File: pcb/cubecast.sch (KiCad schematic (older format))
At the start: 17 parts, among them P1 TP, U1 bq24040, U2 tps62200, U3 ESP-07v2

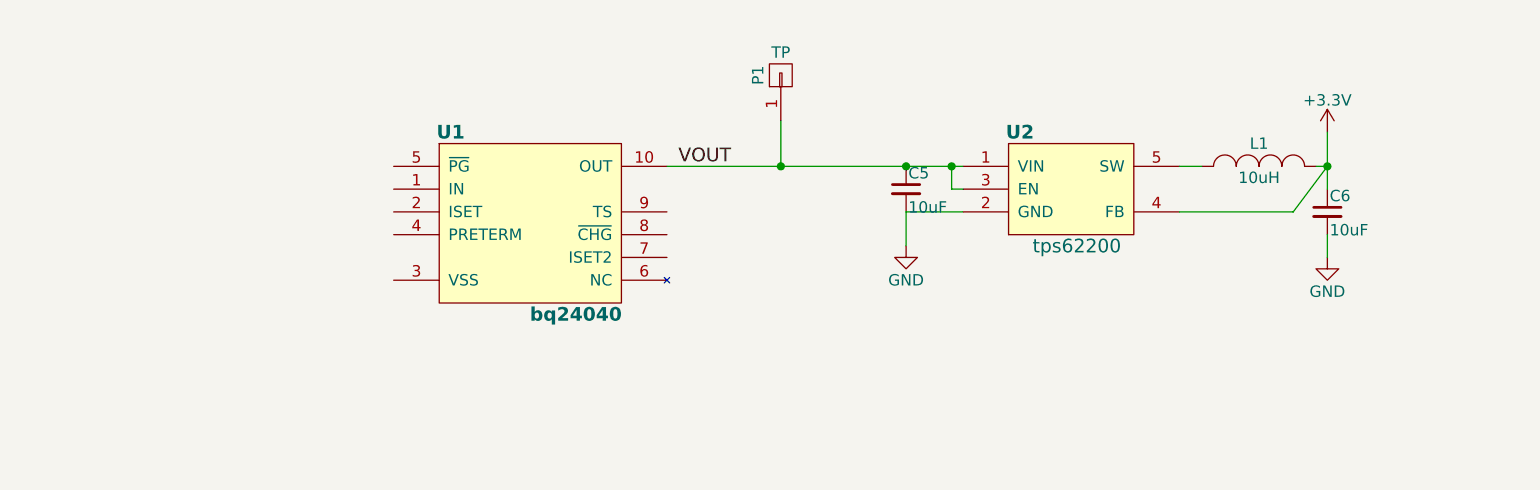
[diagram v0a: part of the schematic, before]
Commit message: footprint for charger
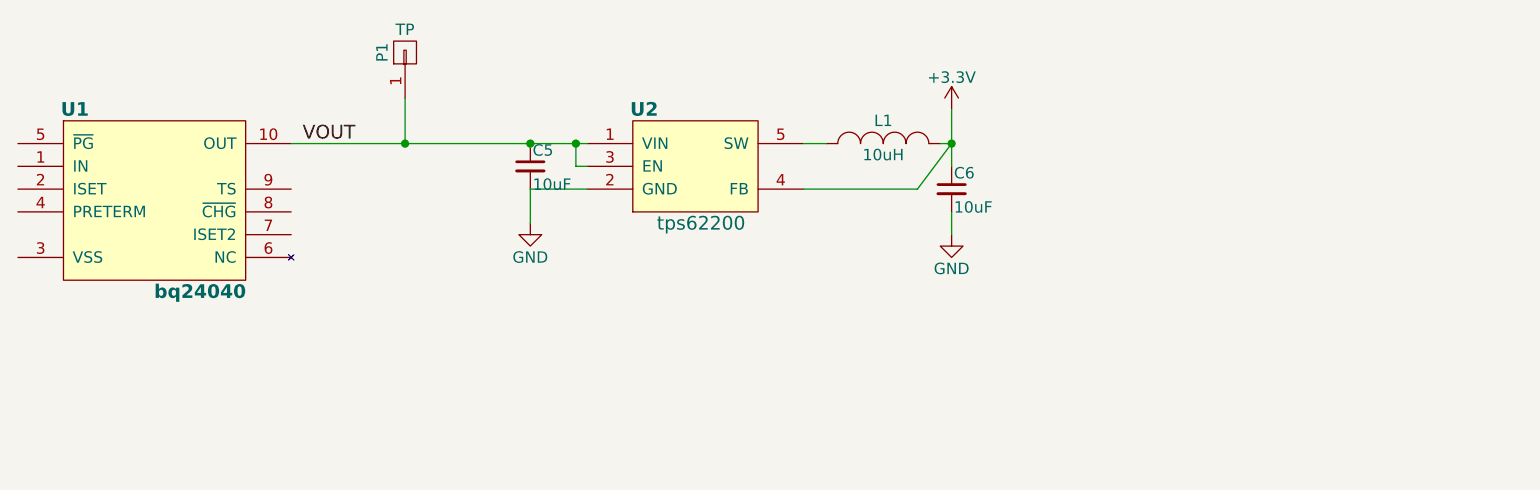
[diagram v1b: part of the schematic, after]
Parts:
- U1: footprint (none) -> SMD:R-PWSON-N10
- U2: footprint (none) -> TO_SOT_Packages_SMD:SOT-23-5
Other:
- moved on the sheet: C5, C6, L1, P1, U1, U2
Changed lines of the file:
@@
 L bq24040 U1
 U 1 1 55C68F96
-P 3550 2450
-F 0 "U1" H 3250 3250 60  0000 C CNB
-F 1 "bq24040" H 3800 2450 60  0000 C CNB
-F 2 "" H 3550 2450 60  0000 C CNN
-F 3 "" H 3550 2450 60  0000 C CNN
-	1    3550 2450
+P 1900 2350
+F 0 "U1" H 1600 3150 60  0000 C CNB
+F 1 "bq24040" H 2150 2350 60  0000 C CNB
+F 2 "SMD:R-PWSON-N10" H 1900 2350 60  0001 C CNN
+F 3 "" H 1900 2350 60  0000 C CNN
+	1    1900 2350
 	1    0    0    -1
 $EndComp
@@
 L tps62200 U2
 U 1 1 55C6910F
-P 6000 1900
-F 0 "U2" H 5750 2150 60  0000 C CNB
-F 1 "tps62200" H 6000 1650 60  0000 C CNN
-F 2 "" H 6000 1900 60  0000 C CNN
-F 3 "" H 6000 1900 60  0000 C CNN
-	1    6000 1900
+P 4350 1800
+F 0 "U2" H 4100 2050 60  0000 C CNB
+F 1 "tps62200" H 4350 1550 60  0000 C CNN
+F 2 "TO_SOT_Packages_SMD:SOT-23-5" H 4350 1800 60  0001 C CNN
+F 3 "" H 4350 1800 60  0000 C CNN
+	1    4350 1800
 	1    0    0    -1
 $EndComp
@@
 L +3.3V #PWR6
 U 1 1 55C693B9
-P 7100 1650
-F 0 "#PWR6" H 7100 1500 50  0001 C CNN
-F 1 "+3.3V" H 7100 1790 50  0000 C CNN
-F 2 "" H 7100 1650 60  0000 C CNN
-F 3 "" H 7100 1650 60  0000 C CNN
-	1    7100 1650
+P 5450 1550
+F 0 "#PWR6" H 5450 1400 50  0001 C CNN
+F 1 "+3.3V" H 5450 1690 50  0000 C CNN
+F 2 "" H 5450 1550 60  0000 C CNN
+F 3 "" H 5450 1550 60  0000 C CNN
+	1    5450 1550
 	1    0    0    -1
 $EndComp
@@
 L INDUCTOR_SMALL L1
 U 1 1 55C693E5
-P 6800 1800
-F 0 "L1" H 6800 1900 50  0000 C CNN
-F 1 "10uH" H 6800 1750 50  0000 C CNN
-F 2 "" H 6800 1800 60  0000 C CNN
-F 3 "" H 6800 1800 60  0000 C CNN
-	1    6800 1800
+P 5150 1700
+F 0 "L1" H 5150 1800 50  0000 C CNN
+F 1 "10uH" H 5150 1650 50  0000 C CNN
+F 2 "" H 5150 1700 60  0000 C CNN
+F 3 "" H 5150 1700 60  0000 C CNN
+	1    5150 1700
 	1    0    0    -1
 $EndComp
@@
 L C_Small C6
 U 1 1 55C694BC
-P 7100 2000
-F 0 "C6" H 7110 2070 50  0000 L CNN
-F 1 "10uF" H 7110 1920 50  0000 L CNN
-F 2 "Capacitors_SMD:C_0603_HandSoldering" H 7100 2000 60  0001 C CNN
-F 3 "" H 7100 2000 60  0000 C CNN
-	1    7100 2000
+P 5450 1900
+F 0 "C6" H 5460 1970 50  0000 L CNN
+F 1 "10uF" H 5460 1820 50  0000 L CNN
+F 2 "Capacitors_SMD:C_0603_HandSoldering" H 5450 1900 60  0001 C CNN
+F 3 "" H 5450 1900 60  0000 C CNN
+	1    5450 1900
 	1    0    0    -1
 $EndComp
 Wire Wire Line
-	6450 1800 6550 1800
+	4800 1700 4900 1700
 Wire Wire Line
-	7050 1800 7100 1800
+	5400 1700 5450 1700
 Wire Wire Line
-	7100 1650 7100 1900
-Connection ~ 7100 1800
+	5450 1550 5450 1800
+Connection ~ 5450 1700
 Wire Wire Line
-	7100 2100 7100 2200
+	5450 2000 5450 2100
 Wire Wire Line
-	6450 2000 6950 2000
+	4800 1900 5300 1900
 Wire Wire Line
-	6950 2000 7100 1800
+	5300 1900 5450 1700
 Wire Wire Line
-	5500 1900 5450 1900
+	3850 1800 3800 1800
 Wire Wire Line
-	5450 1900 5450 1800
-Connection ~ 5450 1800
+	3800 1800 3800 1700
+Connection ~ 3800 1700
 Wire Wire Line
-	4700 1600 4700 1800
-Connection ~ 4700 1800
+	3050 1500 3050 1700
+Connection ~ 3050 1700
 $Comp
 L CONN_01X01 P1
 U 1 1 55C699CD
-P 4700 1400
-F 0 "P1" H 4700 1500 50  0000 C CNN
-F 1 "TP" V 4800 1400 50  0000 C CNN
-F 2 "" H 4700 1400 60  0000 C CNN
-F 3 "" H 4700 1400 60  0000 C CNN
-	1    4700 1400
+P 3050 1300
+F 0 "P1" H 3050 1400 50  0000 C CNN
+F 1 "TP" V 3150 1300 50  0000 C CNN
+F 2 "" H 3050 1300 60  0000 C CNN
+F 3 "" H 3050 1300 60  0000 C CNN
+	1    3050 1300
 	0    -1   -1   0
 $EndComp
-Text Label 4250 1800 0    60   ~ 0
+Text Label 2600 1700 0    60   ~ 0
 VOUT
 $Comp
 L GND #PWR5
 U 1 1 55C69B22
-P 5250 2150
-F 0 "#PWR5" H 5250 1900 50  0001 C CNN
-F 1 "GND" H 5250 2000 50  0000 C CNN
-F 2 "" H 5250 2150 60  0000 C CNN
-F 3 "" H 5250 2150 60  0000 C CNN
-	1    5250 2150
+P 3600 2050
+F 0 "#PWR5" H 3600 1800 50  0001 C CNN
+F 1 "GND" H 3600 1900 50  0000 C CNN
+F 2 "" H 3600 2050 60  0000 C CNN
+F 3 "" H 3600 2050 60  0000 C CNN
+	1    3600 2050
 	1    0    0    -1
 $EndComp
@@
 L C_Small C5
 U 1 1 55C69C7F
-P 5250 1900
-F 0 "C5" H 5260 1970 50  0000 L CNN
-F 1 "10uF" H 5260 1820 50  0000 L CNN
-F 2 "Capacitors_SMD:C_0603_HandSoldering" H 5250 1900 60  0001 C CNN
-F 3 "" H 5250 1900 60  0000 C CNN
-	1    5250 1900
+P 3600 1800
+F 0 "C5" H 3610 1870 50  0000 L CNN
+F 1 "10uF" H 3610 1720 50  0000 L CNN
+F 2 "Capacitors_SMD:C_0603_HandSoldering" H 3600 1800 60  0001 C CNN
+F 3 "" H 3600 1800 60  0000 C CNN
+	1    3600 1800
 	1    0    0    -1
 $EndComp
 Wire Wire Line
-	4200 1800 5500 1800
-Connection ~ 5250 1800
+	2550 1700 3850 1700
+Connection ~ 3600 1700
 Wire Wire Line
-	5500 2000 5250 2000
+	3850 1900 3600 1900
 Wire Wire Line
-	5250 2000 5250 2150
+	3600 1900 3600 2050
 $Comp
 L ESP-07v2 U3
@@
 L GND #PWR7
 U 1 1 55C698DC
-P 7100 2200
-F 0 "#PWR7" H 7100 1950 50  0001 C CNN
-F 1 "GND" H 7100 2050 50  0000 C CNN
-F 2 "" H 7100 2200 60  0000 C CNN
-F 3 "" H 7100 2200 60  0000 C CNN
-	1    7100 2200
+P 5450 2100
+F 0 "#PWR7" H 5450 1850 50  0001 C CNN
+F 1 "GND" H 5450 1950 50  0000 C CNN
+F 2 "" H 5450 2100 60  0000 C CNN
+F 3 "" H 5450 2100 60  0000 C CNN
+	1    5450 2100
 	1    0    0    -1
 $EndComp
